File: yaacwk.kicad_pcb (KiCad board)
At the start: 2 copper layers, 110 x 78 mm, 76 parts, among them IC1 ATMEGA644P-P, IC2 TLP627-2, J1 EXT_PWR, J2 AUDIO_IN, J3 TX_PTT, J4 TX_KEY, J5 PADDLES, J6 TTL_SERIAL, J7 HEADER_6, J8 HEADER_11, J9 PWR_SEL, SW1 SW_PUSH, SW2 SW_PUSH, SW3 SW_PUSH, SW4 SW_PUSH, SW5 SW_PUSH, SW6 SW_PUSH, SW7 SW_PUSH, SW8 SW_PUSH, SW9 SW_PUSH, U1 LM7805, U2 LM2937, Y1 Crystal 16 MHz

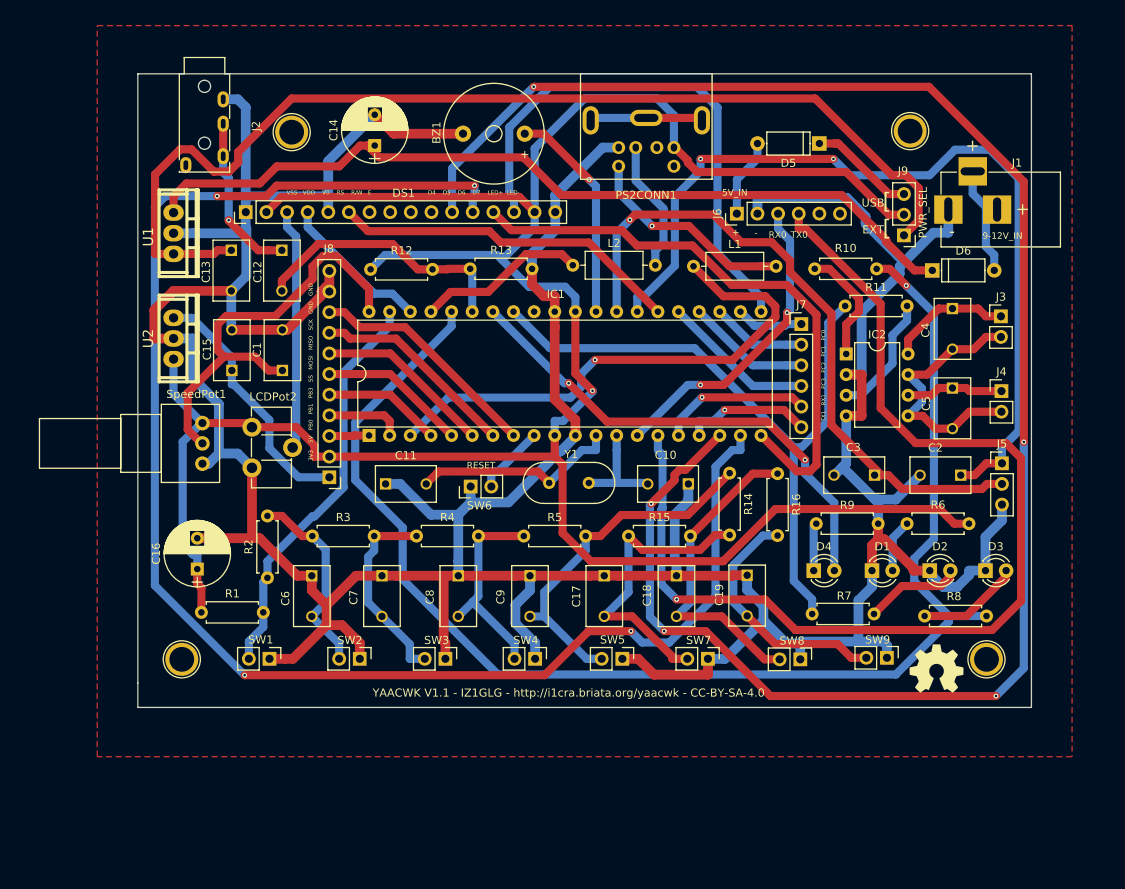
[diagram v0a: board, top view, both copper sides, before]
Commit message: Yaacwk v1.2 with gerber
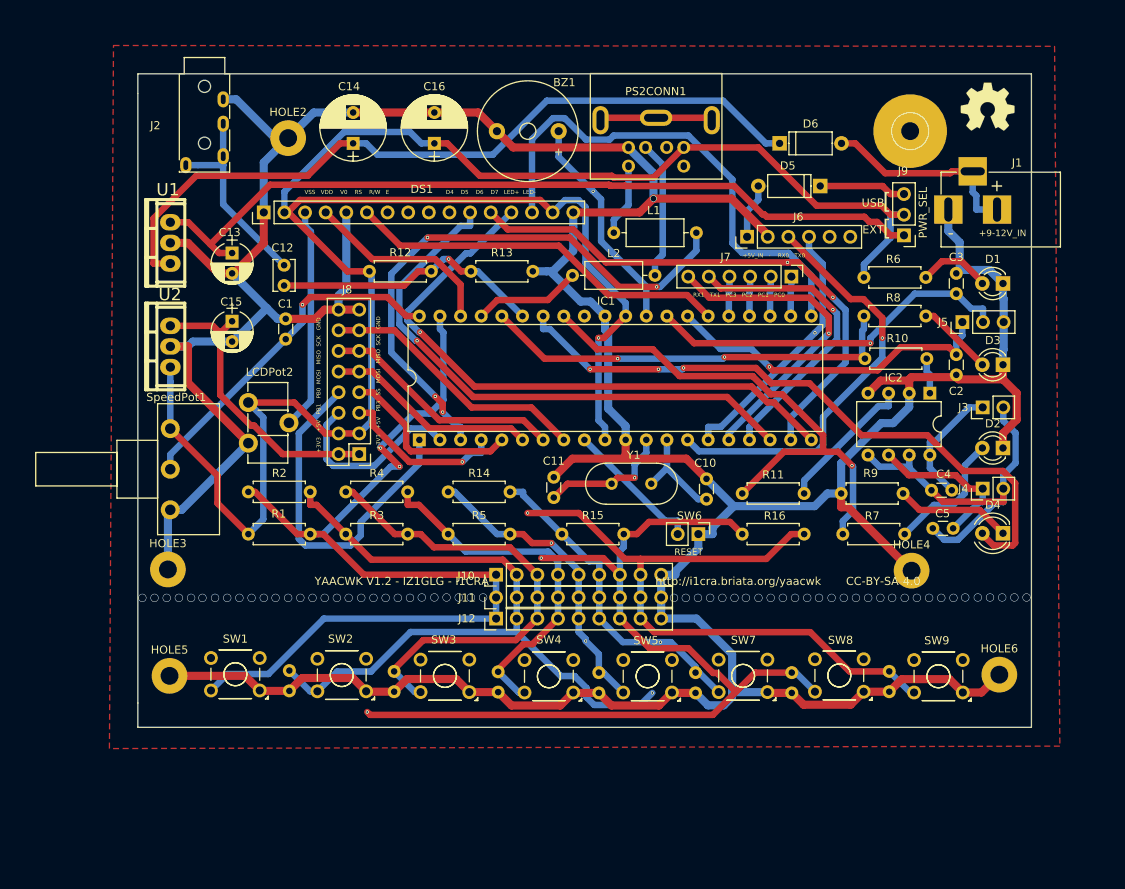
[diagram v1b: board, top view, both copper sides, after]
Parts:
- removed HOLE0: 1pin, Connect:1pin
- added HOLE4: MountingHole_2.2mm_M2_Pad, Mounting_Holes:MountingHole_2.2mm_M2_Pad, F.Cu at (195.2, 117.1)
- added HOLE5: MountingHole_2.2mm_M2_Pad, Mounting_Holes:MountingHole_2.2mm_M2_Pad, F.Cu at (103.9, 130.1)
- added HOLE6: MountingHole_2.2mm_M2_Pad, Mounting_Holes:MountingHole_2.2mm_M2_Pad, F.Cu at (206.1, 129.9)
- added J10: HEADER_9, Pin_Headers:Pin_Header_Straight_1x09_Pitch2.54mm, F.Cu at (144.1, 117.6)
- added J11: HEADER_9, Pin_Headers:Pin_Header_Straight_1x09_Pitch2.54mm, F.Cu at (144.1, 120.4)
- added J12: HEADER_9, Pin_Headers:Pin_Header_Straight_1x09_Pitch2.54mm, F.Cu at (144.1, 123.0)
- C1, C10, C11, C2, C3, C4, C5: footprint Capacitors_ThroughHole:C_Disc_D7.5_P5 -> Capacitors_THT:C_Disc_D3.0mm_W1.6mm_P2.50mm
- C12: footprint Capacitors_ThroughHole:C_Disc_D7.5_P5 -> Capacitors_THT:C_Disc_D3.8mm_W2.6mm_P2.50mm
- C13, C15: value 220nF -> 22uF; footprint Capacitors_ThroughHole:C_Disc_D7.5_P5 -> Capacitors_THT:CP_Radial_D5.0mm_P2.50mm
- C17, C18, C19, C6, C7, C8, C9: footprint Capacitors_ThroughHole:C_Disc_D7.5_P5 -> Capacitors_THT:C_Disc_D3.4mm_W2.1mm_P2.50mm; moved to B.Cu
- D4: footprint LEDs:LED_D3.0mm -> LEDs:LED_D4.0mm
- HOLE2, HOLE3: value 1pin -> MountingHole_2.2mm_M2_Pad; footprint Connect:1pin -> Mounting_Holes:MountingHole_2.2mm_M2_Pad
- J8: value HEADER_11 -> HEADER_8x2; footprint Pin_Headers:Pin_Header_Straight_1x11_Pitch2.54mm -> Pin_Headers:Pin_Header_Straight_2x08_Pitch2.54mm
- R6, R7, R8: value 470 Ohm -> 1kOhm
- R9: value 220 Ohm -> 220Ohm
- SW1, SW2, SW3, SW4, SW5, SW7, SW8, SW9: footprint Pin_Headers:Pin_Header_Straight_1x02_Pitch2.54mm -> Buttons_Switches_THT:SW_TH_Tactile_Omron_B3F-10xx
- SpeedPot1: footprint Potentiometers:Potentiometer_Alps_RK097_Single_Vertical -> Potentiometers:Potentiometer_Piher_T16H_Single_Vertical
- moved HOLE2 107.3 mm to (118.5, 63.9)
- moved REF*** 69.4 mm to (204.6, 60.0)
- moved C16 60.0 mm to (136.5, 64.5)
- moved D1 38.8 mm to (206.5, 81.8), turned to 180 degrees
- moved R8 36.9 mm to (197.0, 85.8), turned to 180 degrees
- moved R14 34.7 mm to (138.2, 107.4), turned to 0 degrees
- moved R6 30.4 mm to (197.0, 81.0), turned to 180 degrees
- moved SW6 28.6 mm to (169.0, 112.6), turned to 270 degrees
- moved R11 26.3 mm to (174.4, 107.6)
- moved D3 25.4 mm to (206.5, 91.8), turned to 180 degrees
- moved C3 24.5 mm to (200.8, 83.0), turned to 90 degrees
- moved D6 24.5 mm to (179.0, 64.5)
- moved D4 23.8 mm to (206.5, 112.5), turned to 180 degrees
- moved C19 22.6 mm to (192.5, 132.0), turned to 90 degrees
- moved C4 22.4 mm to (200.2, 107.2), turned to 180 degrees
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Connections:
- DS1 pad 10: Net-(DS1-Pad10) -> (no net)
- DS1 pad 7: Net-(DS1-Pad7) -> (no net)
- DS1 pad 8: Net-(DS1-Pad8) -> (no net)
- DS1 pad 9: Net-(DS1-Pad9) -> (no net)
- HOLE2 pad 1: (no net) -> GND
- HOLE3 pad 1: (no net) -> GND
- IC1 pad 32: Net-(IC1-Pad32) -> (no net)
- J2 pad 5: Net-(J2-Pad5) -> Net-(C12-Pad1)
- J6 pad 5: Net-(J6-Pad5) -> (no net)
- J6 pad 6: Net-(J6-Pad6) -> (no net)
- J7 pad 5: Net-(IC1-Pad16) -> Net-(IC1-Pad17)
- J7 pad 6: Net-(IC1-Pad17) -> Net-(IC1-Pad16)
- J8 pad 10: GND -> Net-(IC1-Pad6)
- J8 pad 11: GND -> Net-(IC1-Pad7)
- J8 pad 2: Net-(C16-Pad1) -> Net-(C15-Pad1)
- J8 pad 3: Net-(IC1-Pad1) -> Net-(C16-Pad1)
- J8 pad 4: Net-(IC1-Pad2) -> Net-(C16-Pad1)
- J8 pad 6: Net-(IC1-Pad5) -> Net-(IC1-Pad2)
- J8 pad 7: Net-(IC1-Pad6) -> Net-(IC1-Pad5)
- J8 pad 8: Net-(IC1-Pad7) -> Net-(IC1-Pad1)
- J8 pad 9: Net-(IC1-Pad8) -> Net-(IC1-Pad6)
- PS2CONN1 pad 2: Net-(PS2CONN1-Pad2) -> (no net)
- PS2CONN1 pad 6: Net-(PS2CONN1-Pad6) -> (no net)
- U2 pad VI: Net-(C15-Pad1) -> Net-(C16-Pad1)
- U2 pad VO: Net-(C16-Pad1) -> Net-(C15-Pad1)
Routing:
- net Net-(DS1-Pad11): track 222.5 -> 69.6 mm, vias 5 -> 1
- net Net-(DS1-Pad12): track 190.9 -> 67.4 mm, vias 4 -> 2
- net Net-(IC1-Pad36): track 169.7 -> 52.5 mm, vias 1 -> 2
- net Net-(IC1-Pad15): track 132.7 -> 32.5 mm
- net Net-(C18-Pad2): track 39.4 -> 113.4 mm, vias 0 -> 2
- net Net-(IC1-Pad39): track 50.1 -> 117.4 mm, vias 0 -> 20
- net Net-(C6-Pad2): track 24.4 -> 91.5 mm, vias 0 -> 21
- net Net-(C2-Pad1): track 106.8 -> 41.7 mm, vias 2 -> 1
- net Net-(C19-Pad2): track 30.7 -> 82.4 mm, vias 0 -> 1
- net Net-(C16-Pad1): track 303.1 -> 263.2 mm
- net Net-(IC1-Pad1): track 4.92 -> 43.3 mm
- net Net-(C3-Pad1): track 82.0 -> 45.6 mm
- net Net-(C7-Pad2): track 24.6 -> 58.0 mm
- net Net-(C13-Pad1): track 131.4 -> 100.2 mm
- net Net-(IC1-Pad17): track 15.8 -> 37.7 mm
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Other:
- board size 110 x 78 mm -> 110 x 80.4 mm
- net class Default: clearance 0.4 -> 0.2; trace_width 1 -> 0.8; via_dia 0.6 -> 0.4; via_drill 0.4 -> 0.3
- net class gnd: clearance 0.5 -> 0.25; trace_width 1.2 -> 1; via_dia 0.6 -> 0.8; via_drill 0.4 -> 0.7
- rule trace_clearance: 0.4 -> 0.2
- rule trace_min: 0.2 -> 0.4
- board text added: "+3V3 +5V PB1 PB0 MOSI MISO SCK GND"
- board text added: "+3V3 +5V PB3 SS MOSI MISO SCK GND"
- board text added: "+5V_IN - RX0 TX0"
- board text added: "+9-12V_IN"
- board text added: "RX1 TX1 PC3 PC2 PC1 PC0"
- board text added: "YAACWK V1.2 - IZ1GLG - I1CRA http://i1cra.briata.org/yaacwk CC-BY-SA-4.0"
- board text removed: "3V3 5V PB0 PB1 PB3 SS MOSI MISO SCK GND GND"
- board text removed: "5V_IN"
- board text removed: "9-12V_IN"
- board text removed: "RX0"
- board text removed: "TX0"
- board text removed: "TX1 RX1 PC3 PC2 PC1 PC0"
- board text removed: "YAACWK V1.1 - IZ1GLG - http://i1cra.briata.org/yaacwk - CC-BY-SA-4.0"

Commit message: Yaacwk v1.3 with gerber and current WIP
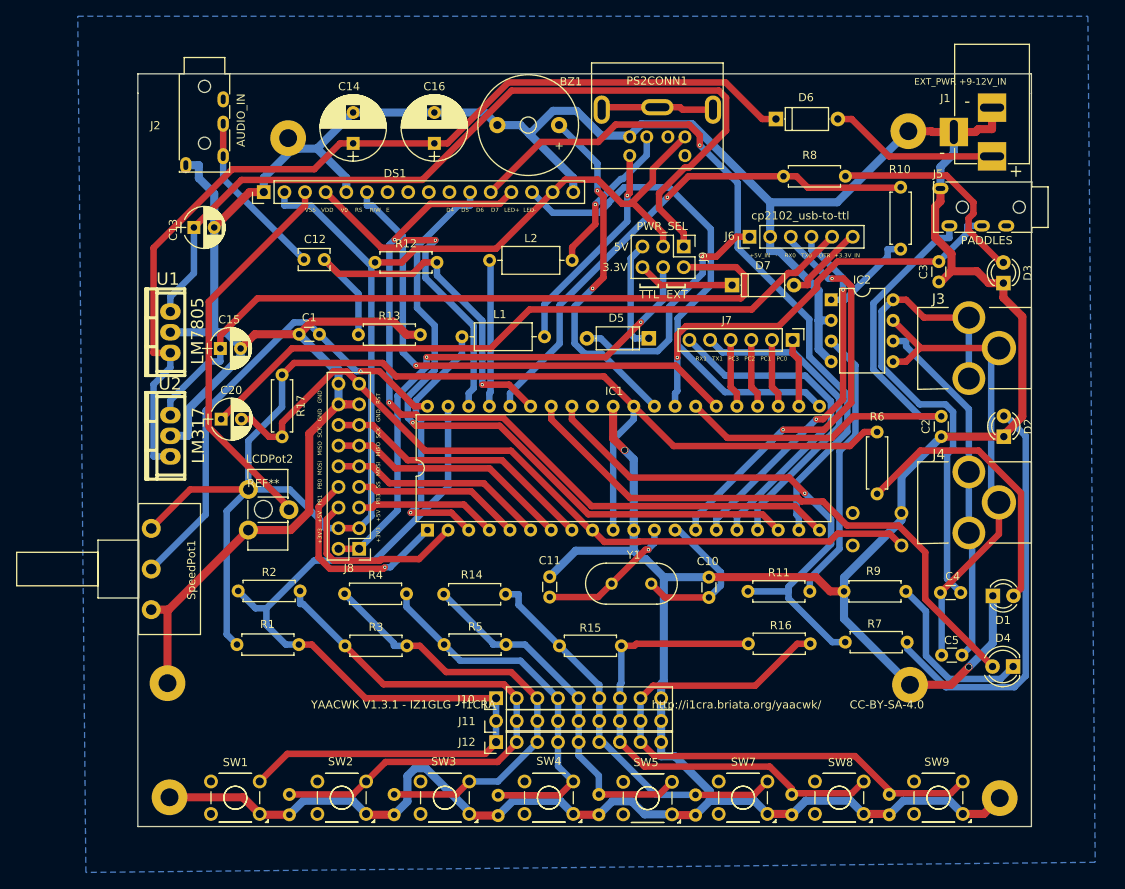
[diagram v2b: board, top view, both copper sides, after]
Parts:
- removed REF***: OSHW-Symbol_6.7x6mm_SilkScreen, Symbols:OSHW-Symbol_6.7x6mm_SilkScreen
- added C20: 0.47uF, Capacitors_THT:CP_Radial_D5.0mm_P2.50mm, F.Cu at (110.2, 98.5)
- added D7: D_ALT, Diodes_THT:D_A-405_P7.62mm_Horizontal, F.Cu at (173.2, 82.0)
- added R17: 10kOhm, Resistors_THT:R_Axial_DIN0207_L6.3mm_D2.5mm_P7.62mm_Horizontal, F.Cu at (117.8, 93.0)
- added REF**: MountingHole_2.2mm_M2, Mounting_Holes:MountingHole_2.2mm_M2, F.Cu at (115.5, 109.5)
- added REF1: KiCad-Logo_8mm_SilkScreen, Symbols:KiCad-Logo_8mm_SilkScreen, B.Cu at (172.2, 103.7)
- added REF2: OSHW-Logo_7.5x8mm_SilkScreen, Symbols:OSHW-Logo_7.5x8mm_SilkScreen, B.Cu at (155.8, 104.2)
- added REF3: Symbol_CreativeCommons_SilkScreenTop_Type2_Big, Symbols:Symbol_CreativeCommons_SilkScreenTop_Type2_Big, B.Cu at (143.6, 103.9)
- HOLE1: value 1pin -> MountingHole_2.2mm_M2_Pad; footprint Connect:1pin -> Mounting_Holes:MountingHole_2.2mm_M2_Pad
- J3, J4: footprint Pin_Headers:Pin_Header_Straight_1x02_Pitch2.54mm -> PJRAN1X1U03AUX
- J5: footprint Pin_Headers:Pin_Header_Straight_1x03_Pitch2.54mm -> PJ320A:PJ320A_3.5mm_4_conductors_audio_plug
- J8: value HEADER_8x2 -> HEADER_9x2; footprint Pin_Headers:Pin_Header_Straight_2x08_Pitch2.54mm -> Pin_Headers:Pin_Header_Straight_2x09_Pitch2.54mm
- J9: footprint Pin_Headers:Pin_Header_Straight_1x03_Pitch2.54mm -> Pin_Headers:Pin_Header_Straight_2x03_Pitch2.54mm
- R9: value 220Ohm -> 220 Ohm
- SW1, SW2, SW3, SW4, SW5, SW7, SW8, SW9: value SW_PUSH -> SW_SPDT
- SW6: value SW_PUSH -> SW_SPDT; footprint Pin_Headers:Pin_Header_Straight_1x02_Pitch2.54mm -> Buttons_Switches_THT:SW_TH_Tactile_Omron_B3F-10xx; moved to B.Cu
- U2: value LM2937 -> LM317
- moved D1 38.5 mm to (205.2, 120.2), turned to 0 degrees
- moved L1 31.6 mm to (139.9, 88.3), turned to 0 degrees
- moved D5 28.2 mm to (162.9, 88.5)
- moved R6 27.3 mm to (191.0, 107.7), turned to 90 degrees
- moved J9 27.1 mm to (167.2, 77.2), turned to 270 degrees
- moved SW6 25.1 mm to (194.0, 110.0), turned to 180 degrees
- moved R10 21.6 mm to (193.9, 69.9), turned to 270 degrees
- moved R8 19.8 mm to (187.1, 68.5)
- moved IC2 16.7 mm to (185.3, 83.8), turned to 0 degrees
- moved J5 16.6 mm to (210.1, 72.3), turned to 180 degrees
- moved D4 16.4 mm to (207.8, 128.9)
- moved R13 15.9 mm to (127.2, 88.0)
- moved C5 15.6 mm to (201.4, 127.5)
- moved C6 15.2 mm to (118.7, 147.2)
- moved HOLE6 15.2 mm to (206.1, 145.1)
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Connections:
- C16 pad 1: Net-(C16-Pad1) -> Net-(C14-Pad1)
- DS1 pad 15: Net-(C16-Pad1) -> Net-(DS1-Pad15)
- DS1 pad 2: Net-(C16-Pad1) -> Net-(DS1-Pad15)
- IC1 pad 10: Net-(C16-Pad1) -> Net-(DS1-Pad15)
- IC1 pad 30: Net-(C16-Pad1) -> Net-(DS1-Pad15)
- IC1 pad 9: Net-(IC1-Pad9) -> Net-(C20-Pad2)
- J1 pad 1: GND -> Net-(D6-Pad2)
- J1 pad 2: Net-(D6-Pad2) -> GND
- J1 pad 3: Net-(D6-Pad2) -> GND
- J2 pad 2: GND -> (no net)
- J2 pad 5: Net-(C12-Pad1) -> GND
- J3 pad 1: Net-(C4-Pad1) -> Net-(C4-Pad2)
- J3 pad 2: Net-(C4-Pad2) -> Net-(C4-Pad1)
- J4 pad 1: Net-(C5-Pad1) -> Net-(C4-Pad2)
- J4 pad 2: Net-(C4-Pad2) -> Net-(C5-Pad1)
- J5 pad 2: Net-(C3-Pad1) -> (no net)
- J5 pad 3: GND -> Net-(C3-Pad1)
- J6 pad 5: (no net) -> Net-(C20-Pad1)
- J6 pad 6: (no net) -> Net-(D7-Pad2)
- J8 pad 1: Net-(C15-Pad1) -> Net-(J8-Pad1)
- J8 pad 2: Net-(C15-Pad1) -> Net-(J8-Pad1)
- J8 pad 3: Net-(C16-Pad1) -> Net-(DS1-Pad15)
- J8 pad 4: Net-(C16-Pad1) -> Net-(DS1-Pad15)
- J9 pad 2: Net-(C16-Pad1) -> Net-(C15-Pad1)
- J9 pad 3: Net-(D5-Pad1) -> Net-(DS1-Pad15)
- LCDPot2 pad 1: Net-(C16-Pad1) -> Net-(DS1-Pad15)
- PS2CONN1 pad 4: Net-(C16-Pad1) -> Net-(DS1-Pad15)
- R1 pad 1: Net-(C16-Pad1) -> Net-(DS1-Pad15)
- R12 pad 1: Net-(C16-Pad1) -> Net-(DS1-Pad15)
- R6 pad 2: Net-(C16-Pad1) -> Net-(DS1-Pad15)
- SW1 pad 2: Net-(IC1-Pad39) -> (no net)
- SW1 pad 3: (no net) -> Net-(IC1-Pad39)
- SW2 pad 2: Net-(C6-Pad2) -> (no net)
- SW2 pad 3: (no net) -> Net-(C6-Pad2)
- SW3 pad 2: Net-(C7-Pad2) -> (no net)
- SW3 pad 3: (no net) -> Net-(C7-Pad2)
- SW4 pad 2: Net-(C8-Pad2) -> (no net)
- SW4 pad 3: (no net) -> Net-(C8-Pad2)
- SW5 pad 2: Net-(C9-Pad2) -> (no net)
- SW5 pad 3: (no net) -> Net-(C9-Pad2)
- SW6 pad 2: Net-(IC1-Pad9) -> (no net)
- SW7 pad 2: Net-(C17-Pad2) -> (no net)
- SW7 pad 3: (no net) -> Net-(C17-Pad2)
- SW8 pad 2: Net-(C18-Pad2) -> (no net)
- SW8 pad 3: (no net) -> Net-(C18-Pad2)
- SW9 pad 2: Net-(C19-Pad2) -> (no net)
- SW9 pad 3: (no net) -> Net-(C19-Pad2)
- SpeedPot1 pad 1: Net-(C16-Pad1) -> Net-(DS1-Pad15)
- U2 pad VI: Net-(C16-Pad1) -> Net-(C14-Pad1)
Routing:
- net Net-(DS1-Pad15): track 0.00 -> 265.4 mm
- net Net-(C16-Pad1): track 263.2 -> 0.00 mm, vias 1 -> 0
- net GND: track 511.8 -> 616.9 mm, vias 1 -> 2
- net Net-(C20-Pad2): track 0.00 -> 96.3 mm
- net Net-(C20-Pad1): track 0.00 -> 84.5 mm
- net Net-(J8-Pad1): track 0.00 -> 65.6 mm, vias 0 -> 2
- net Net-(C15-Pad1): track 36.3 -> 90.0 mm
- net Net-(C18-Pad2): track 113.4 -> 61.4 mm, vias 2 -> 0
- net Net-(C4-Pad1): track 15.3 -> 60.9 mm
- net Net-(IC1-Pad3): track 70.2 -> 32.8 mm, vias 4 -> 1
- net Net-(D2-Pad2): track 16.0 -> 51.2 mm
- net Net-(D1-Pad2): track 9.01 -> 35.1 mm
- net Net-(C2-Pad1): track 41.7 -> 66.0 mm, vias 1 -> 0
- net Net-(C5-Pad1): track 19.9 -> 44.2 mm
- net Net-(C14-Pad1): track 94.0 -> 117.6 mm
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- added copper zone on B.Cu, net GND
- removed copper zone on F.Cu, net GND
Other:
- board size 110 x 80.4 mm -> 110 x 92.7 mm
- board text added: "+3V3 +5V PB1 PB0 MOSI MISO SCK GND GND"
- board text added: "+3V3 +5V PB3 SS MOSI MISO SCK GND RST"
- board text added: "+5V_IN - RX0 TX0 DTR +3.3V_IN"
- board text added: "3.3V"
- board text added: "5V"
- board text added: "AUDIO_IN"
- board text added: "EXT_PWR +9-12V_IN"
- board text added: "PADDLES"
- board text added: "TTL"
- board text added: "YAACWK V1.3.1 - IZ1GLG - I1CRA http://i1cra.briata.org/yaacwk/ CC-BY-SA-4.0"
- board text added: "cp2102_usb-to-ttl"
- board text removed: "+3V3 +5V PB1 PB0 MOSI MISO SCK GND"
- board text removed: "+3V3 +5V PB3 SS MOSI MISO SCK GND"
- board text removed: "+5V_IN - RX0 TX0"
- board text removed: "+9-12V_IN"
- board text removed: "USB"
- board text removed: "YAACWK V1.2 - IZ1GLG - I1CRA http://i1cra.briata.org/yaacwk CC-BY-SA-4.0"
